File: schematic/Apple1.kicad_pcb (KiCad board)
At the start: 2 copper layers, 162.8 x 120.7 mm, 65 parts, among them J1 RCJ-041, J2 USB_A, J4 PWR, J5 ARM_JTAG_SWD, J6 SLOT, J7 EDGE, J8 12V, J9 -12V, SW1 RST, SW2 CLEAR, SW3 PWR, U1 WD65C02, U10 L7805, U2 6821 (W65C21N), U3 ATSAMD21E18A-A, U4 74LS138, U5 AT28C64B-15PU, U6 AS6C62256, U7 74HC00, U9 LD33CV

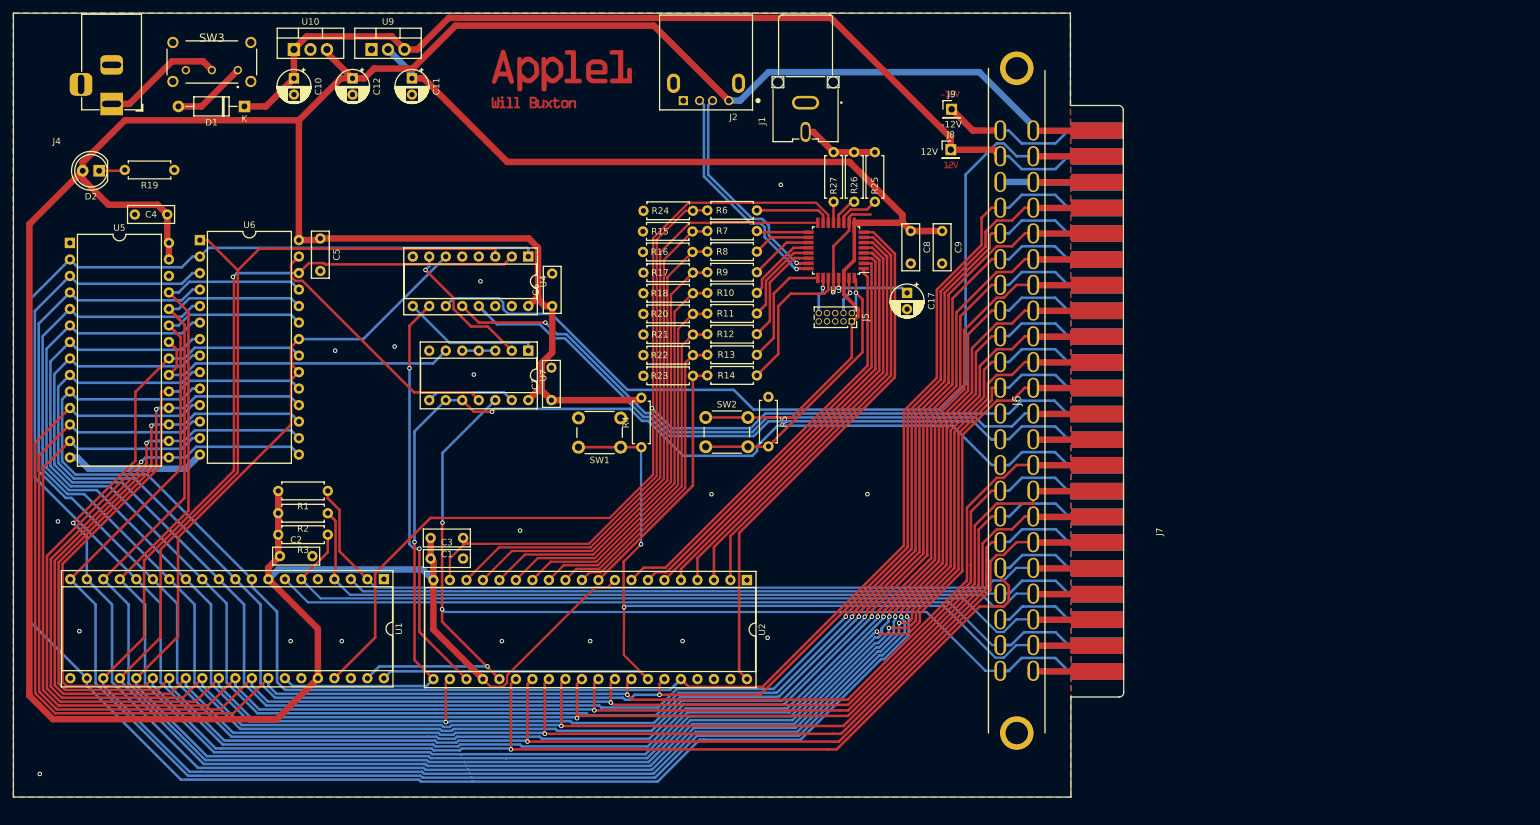
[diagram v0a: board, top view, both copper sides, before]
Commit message: rpi final
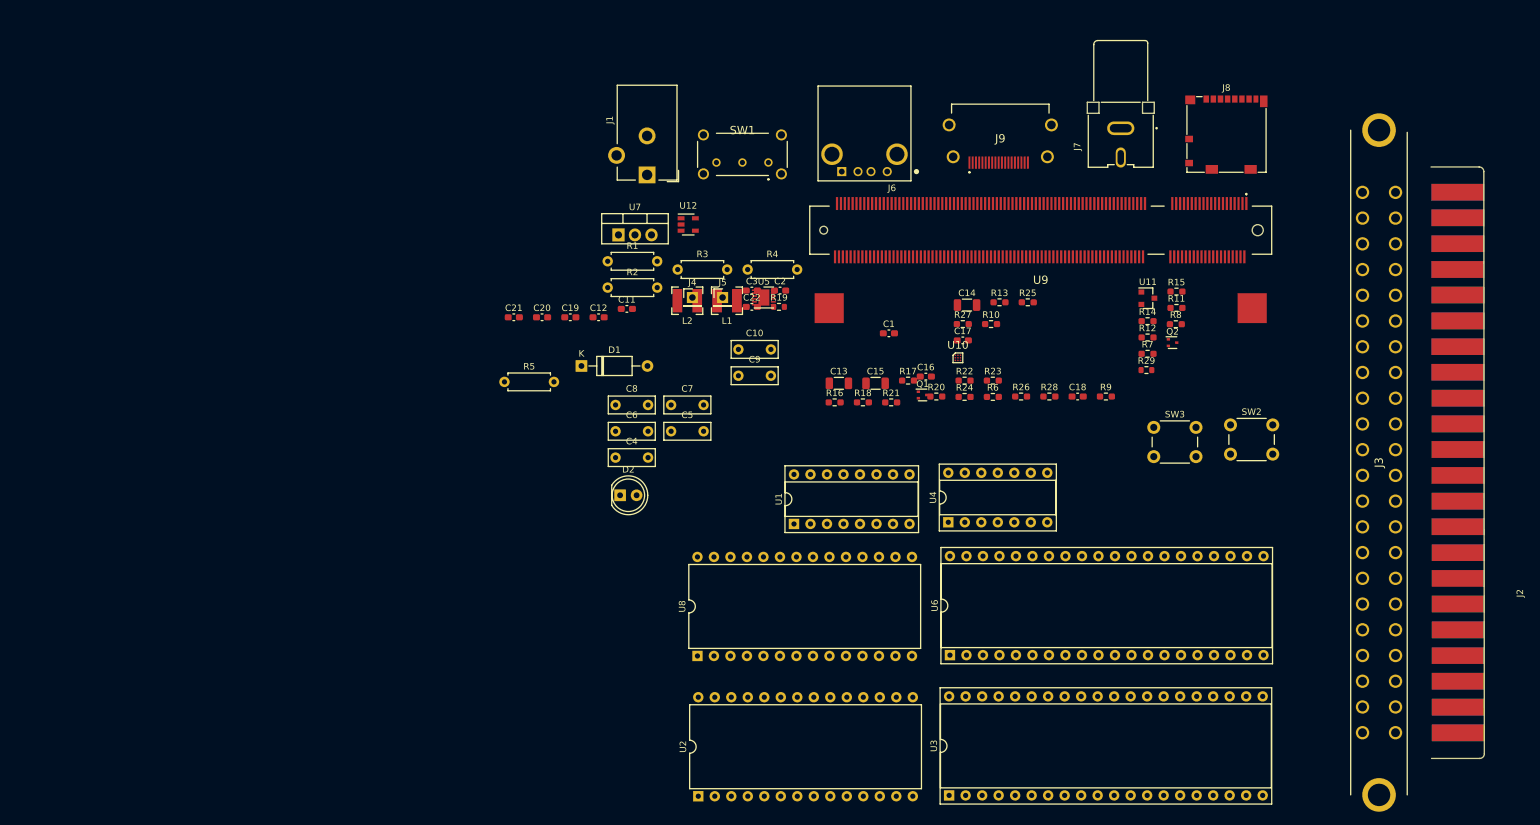
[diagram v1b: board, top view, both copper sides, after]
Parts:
- removed G***: LOGO, Apple1Title:n12v
- removed G***: LOGO, Apple1Title:12v
- removed G***: LOGO, Title:title
- added C13: 47uF, Capacitor_SMD:C_1206_3216Metric, F.Cu at (158.8, 74.6)
- added C14: 47uF, Capacitor_SMD:C_1206_3216Metric, F.Cu at (178.5, 62.6)
- added C15: 47uF, Capacitor_SMD:C_1206_3216Metric, F.Cu at (164.4, 74.6)
- added C16: 4.7uF, Capacitor_SMD:C_0603_1608Metric_Pad1.08x0.95mm_HandSolder, F.Cu at (172.2, 73.6)
- added C18: 0.1uF, Capacitor_SMD:C_0603_1608Metric_Pad1.08x0.95mm_HandSolder, F.Cu at (195.5, 76.7)
- added C19: 10uF, Capacitor_SMD:C_0603_1608Metric_Pad1.08x0.95mm_HandSolder, F.Cu at (117.5, 64.5)
- added C20: 10uF, Capacitor_SMD:C_0603_1608Metric_Pad1.08x0.95mm_HandSolder, F.Cu at (113.1, 64.5)
- added C21: 0.47uF, Capacitor_SMD:C_0603_1608Metric_Pad1.08x0.95mm_HandSolder, F.Cu at (108.8, 64.5)
- added C22: 0.47uF, Capacitor_SMD:C_0603_1608Metric_Pad1.08x0.95mm_HandSolder, F.Cu at (145.4, 62.9)
- added J3: SLOT, 307-044-520-202:307044520202, F.Cu at (244.5, 128.4)
- added L1: 4.7uH, Inductor_SMD:L_Bourns-SRN4018, F.Cu at (141.6, 61.9)
- added L2: 4.7uH, Inductor_SMD:L_Bourns-SRN4018, F.Cu at (135.5, 61.9)
- added Q1: DMG1012T, Package_TO_SOT_SMD:SOT-523, F.Cu at (171.7, 76.4)
- added Q2: DMG1012T, Package_TO_SOT_SMD:SOT-523, F.Cu at (210.2, 68.4)
- added R28: 2k, Resistor_SMD:R_0603_1608Metric_Pad0.98x0.95mm_HandSolder, F.Cu at (191.2, 76.7)
- added R29: 100k, Resistor_SMD:R_0603_1608Metric, F.Cu at (206.1, 72.6)
- added U11: AP2331W, Package_TO_SOT_SMD:SOT-23, F.Cu at (206.4, 61.5)
- added U12: AP7315DQ-2.5, Package_TO_SOT_SMD:SOT-23-5, F.Cu at (135.6, 50.2)
- added U8: AT28C64B-15PU, Package_DIP:DIP-28_W15.24mm, F.Cu at (137.0, 116.6)
- C1: value 0.01uF -> 0.33uF; footprint Capacitor_THT:C_Rect_L7.0mm_W2.5mm_P5.00mm -> Capacitor_SMD:C_0603_1608Metric_Pad1.08x0.95mm_HandSolder
- C10: value 10uF -> 0.1uF; footprint Capacitor_THT:CP_Radial_D5.0mm_P2.50mm -> Capacitor_THT:C_Rect_L7.0mm_W2.5mm_P5.00mm
- C11: footprint Capacitor_THT:CP_Radial_D5.0mm_P2.50mm -> Capacitor_SMD:C_0603_1608Metric_Pad1.08x0.95mm_HandSolder
- C12: value 1uF -> 10uF; footprint Capacitor_THT:CP_Radial_D5.0mm_P2.50mm -> Capacitor_SMD:C_0603_1608Metric_Pad1.08x0.95mm_HandSolder
- C17: value 1uF -> 0.1uF; footprint Capacitor_THT:CP_Radial_D5.0mm_P2.50mm -> Capacitor_SMD:C_0603_1608Metric_Pad1.08x0.95mm_HandSolder
- C2, C3: footprint Capacitor_THT:C_Rect_L7.0mm_W2.5mm_P5.00mm -> Capacitor_SMD:C_0603_1608Metric_Pad1.08x0.95mm_HandSolder
- C4: value 0.1uF -> 0.01uF
- J1: value RCJ-041 -> PWR; footprint CUI_RCJ-041 -> Connector_BarrelJack:BarrelJack_CUI_PJ-102AH_Horizontal
- J2: value USB_A -> EDGE; footprint UJ2-AH-4-TH:CUI_UJ2-AH-4-TH -> Connector_PCBEdge:EDAC_Edge_307-044-520-202
- J4: value PWR -> 12V; footprint Connector_BarrelJack:BarrelJack_Horizontal -> Connector_PinHeader_2.54mm:PinHeader_1x01_P2.54mm_Vertical
- J5: value ARM_JTAG_SWD -> -12V; footprint Connector_PinSocket_1.27mm:PinSocket_2x05_P1.27mm_Vertical -> Connector_PinHeader_2.54mm:PinHeader_1x01_P2.54mm_Vertical
- J6: value SLOT -> USB_A; footprint 307-044-520-202:307044520202 -> UJ2-AH-4-TH:CUI_UJ2-AH-4-TH
- J7: value EDGE -> RCJ-041; footprint Connector_PCBEdge:EDAC_Edge_307-044-520-202 -> CUI_RCJ-041
- J8: value 12V -> Micro_SD_Card_Det; footprint Connector_PinHeader_2.54mm:PinHeader_1x01_P2.54mm_Vertical -> Connector_Card:microSD_HC_Molex_104031-0811
- J9: value -12V -> HDMI_A; footprint Connector_PinHeader_2.54mm:PinHeader_1x01_P2.54mm_Vertical -> 10029449-111RLF:10029449111RLF
- R10, R11, R12, R13, R14, R6, R7, R8, R9: value 1K -> 2k; footprint Resistor_THT:R_Axial_DIN0207_L6.3mm_D2.5mm_P7.62mm_Horizontal -> Resistor_SMD:R_0603_1608Metric_Pad0.98x0.95mm_HandSolder
- R15, R16, R17, R18, R20, R21, R22, R23, R24: value 2k -> 1K; footprint Resistor_THT:R_Axial_DIN0207_L6.3mm_D2.5mm_P7.62mm_Horizontal -> Resistor_SMD:R_0603_1608Metric_Pad0.98x0.95mm_HandSolder
- R19: value 330 -> 100k; footprint Resistor_THT:R_Axial_DIN0207_L6.3mm_D2.5mm_P7.62mm_Horizontal -> Resistor_SMD:R_0603_1608Metric
- R25: footprint Resistor_THT:R_Axial_DIN0207_L6.3mm_D2.5mm_P7.62mm_Horizontal -> Resistor_SMD:R_0603_1608Metric_Pad0.98x0.95mm_HandSolder
- R26: value 560 -> 100k; footprint Resistor_THT:R_Axial_DIN0207_L6.3mm_D2.5mm_P7.62mm_Horizontal -> Resistor_SMD:R_0603_1608Metric_Pad0.98x0.95mm_HandSolder
- R27: value 220 -> 100k; footprint Resistor_THT:R_Axial_DIN0207_L6.3mm_D2.5mm_P7.62mm_Horizontal -> Resistor_SMD:R_0603_1608Metric_Pad0.98x0.95mm_HandSolder
- R5: value 3.3K -> 330
- SW1: value RST -> PWR; footprint Button_Switch_THT:SW_PUSH_6mm -> EG1224:EG1224
- SW2: value CLEAR -> RST
- SW3: value PWR -> CLEAR; footprint EG1224:EG1224 -> Button_Switch_THT:SW_PUSH_6mm
- U1: value WD65C02 -> 74LS138; footprint Package_DIP:DIP-40_W15.24mm_Socket -> Package_DIP:DIP-16_W7.62mm_Socket
- U10: value L7805 -> ESD5384; footprint Package_TO_SOT_THT:TO-220-3_Vertical -> SW-On-Semi:WLCSP9-1.14x1.14mm
- U2: value 6821 (W65C21N) -> AS6C62256; footprint Package_DIP:DIP-40_W15.24mm_Socket -> Package_DIP:DIP-28_W15.24mm
- U3: value ATSAMD21E18A-A -> WD65C02; footprint Package_QFP:TQFP-32_7x7mm_P0.8mm -> Package_DIP:DIP-40_W15.24mm_Socket
- U4: value 74LS138 -> 74HC00; footprint Package_DIP:DIP-16_W7.62mm_Socket -> Package_DIP:DIP-14_W7.62mm_Socket
- U5: value AT28C64B-15PU -> PAM2306AYPKE; footprint Package_DIP:DIP-28_W15.24mm -> Package_DFN_QFN:WDFN-12-1EP_3x3mm_P0.45mm_EP1.7x2.5mm
- U6: value AS6C62256 -> 6821 (W65C21N); footprint Package_DIP:DIP-28_W15.24mm -> Package_DIP:DIP-40_W15.24mm_Socket
- U7: value 74HC00 -> L7805; footprint Package_DIP:DIP-14_W7.62mm_Socket -> Package_TO_SOT_THT:TO-220-3_Vertical
- U9: value LD33CV -> RaspberryPi-CM3+L; footprint Package_TO_SOT_THT:TO-220-3_Vertical -> 1717254-4:17172544
- moved SW3 151.3 mm to (207.3, 81.4), turned to 0 degrees
- moved J2 143.0 mm to (263.1, 106.9), turned to 90 degrees
- moved U6 131.9 mm to (175.9, 116.5), turned to 90 degrees
- moved U10 112.7 mm to (177.1, 70.7)
- moved U5 107.1 mm to (147.3, 61.4)
- moved U9 106.7 mm to (189.9, 51.1)
- moved R19 95.4 mm to (149.6, 62.9), turned to 0 degrees
- moved D2 94.5 mm to (125.1, 91.9), turned to 0 degrees
- moved J4 94.2 mm to (136.3, 61.4), turned to 0 degrees
- moved C2 87.2 mm to (149.8, 60.3)
- moved U3 85.7 mm to (175.8, 138.0), turned to 90 degrees
- moved R15 82.6 mm to (210.8, 60.5)
- moved SW2 80.8 mm to (219.1, 81.0)
- moved C10 80.1 mm to (143.3, 69.4), turned to 0 degrees
- moved J6 80.1 mm to (166.2, 42.0), turned to 180 degrees
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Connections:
- C1 pad 1: /CB2 -> +12V
- C1 pad 2: VCC -> GND
- C10 pad 1: +12V -> +5V
- C11 pad 1: +3V3 -> +5V
- C12 pad 1: VCC -> +5V
- C17 pad 1: Net-(C17-Pad1) -> +5V
- C2 pad 1: VCC -> GND
- C2 pad 2: GND -> Net-(C2-Pad2)
- C3 pad 1: VCC -> +5V
- C4 pad 1: VCC -> /CB2
- C4 pad 2: GND -> +5V
- C5 pad 1: VCC -> +5V
- C6 pad 1: VCC -> +5V
- C7 pad 1: VCC -> +5V
- C8 pad 1: +3V3 -> +5V
- C9 pad 1: +3V3 -> +5V
- D2 pad 2: VCC -> +5V
- J1 pad 1: GND -> Net-(J1-Pad1)
- J1 pad 2: Net-(J1-Pad2) -> GND
- J2 pad 1: VCC -> /RF
- J2 pad 2: /KEYD- -> /PHI2O
- J2 pad 3: /KEYD+ -> /RESET
- J2 pad 4: GND -> /SYNC
- J2 pad 5: GND -> /NMI
- J4 pad 1: Net-(J4-Pad1) -> +12V
- J5 pad 1: +3V3 -> -12V
- J6 pad 1: /RF -> +5V
- J6 pad 2: /PHI2O -> /RaspberryPi/USB_D-
- J6 pad 3: /RESET -> /RaspberryPi/USB_D+
- J6 pad 4: /SYNC -> GND
- J6 pad 5: /NMI -> GND
- J7 pad 1: /RF -> GND
- J7 pad 2: /PHI2O -> /RaspberryPi/TVDAC
- J8 pad 1: +12V -> /RaspberryPi/SDX_D2
- J9 pad 1: -12V -> /RaspberryPi/HDMI_D2_P
- R1 pad 2: VCC -> +5V
- R10 pad 1: Net-(R10-Pad1) -> GND
- R11 pad 1: Net-(R11-Pad1) -> GND
- R11 pad 2: /PB3 -> /PB5
- R12 pad 1: Net-(R12-Pad1) -> GND
- R12 pad 2: /PB2 -> /PB6
- R13 pad 1: Net-(R13-Pad1) -> GND
- R13 pad 2: /PB1 -> /DA
- R14 pad 1: Net-(R14-Pad1) -> GND
- R14 pad 2: /PB0 -> /CB2
- R15 pad 1: GND -> Net-(R15-Pad1)
- R15 pad 2: /DA -> /RESET
- R16 pad 1: GND -> Net-(R16-Pad1)
- R16 pad 2: /PB6 -> /PB0
- R17 pad 1: GND -> Net-(R17-Pad1)
- R17 pad 2: /PB5 -> /PB1
- R18 pad 1: GND -> Net-(R18-Pad1)
- R18 pad 2: /PB4 -> /PB2
- R19 pad 1: GND -> +5V
- R19 pad 2: Net-(D2-Pad1) -> Net-(C2-Pad2)
- R2 pad 2: VCC -> +5V
- R20 pad 1: GND -> Net-(R20-Pad1)
- R21 pad 1: GND -> Net-(R21-Pad1)
- R21 pad 2: /PB2 -> /PB4
- R22 pad 1: GND -> Net-(R22-Pad1)
- R22 pad 2: /PB1 -> /PB5
- R23 pad 1: GND -> Net-(R23-Pad1)
- R23 pad 2: /PB0 -> /PB6
- R24 pad 1: GND -> Net-(R24-Pad1)
- R24 pad 2: /CB2 -> /DA
- R25 pad 2: Net-(J1-Pad2) -> /CB2
- R26 pad 1: Net-(R26-Pad1) -> /STROBE
- R26 pad 2: Net-(J1-Pad2) -> GND
- R27 pad 1: Net-(R27-Pad1) -> /PA0
- R27 pad 2: Net-(J1-Pad2) -> GND
- R3 pad 2: VCC -> +5V
- R4 pad 2: VCC -> +5V
- R5 pad 2: /SWDIO -> Net-(D2-Pad1)
- R6 pad 1: Net-(R6-Pad1) -> GND
- R6 pad 2: /CB2 -> /PB0
- R7 pad 1: Net-(R7-Pad1) -> GND
- R7 pad 2: /DA -> /PB1
- R8 pad 1: Net-(R8-Pad1) -> GND
- R8 pad 2: /PB6 -> /PB2
- R9 pad 1: Net-(R9-Pad1) -> GND
- R9 pad 2: /PB5 -> /PB3
- SW1 pad 1: /RESET -> Net-(D1-Pad2)
- SW1 pad 2: GND -> Net-(J1-Pad1)
- SW2 pad 1: +3V3 -> /RESET
- SW2 pad 2: /SWDIO -> GND
- SW3 pad 1: Net-(D1-Pad2) -> GND
- SW3 pad 2: Net-(J4-Pad1) -> /RaspberryPi/CLEAR
- U1 pad 1: (no net) -> /A12
- U1 pad 10: /A1 -> /$D000
- U1 pad 11: /A2 -> /$C000
- U1 pad 12: /A3 -> /$B000
- U1 pad 13: /A4 -> /$A000
- U1 pad 14: /A5 -> (no net)
- U1 pad 15: /A6 -> (no net)
- U1 pad 16: /A7 -> +5V
- U1 pad 2: /RDY -> /A13
- U1 pad 3: /PHI1O -> /A14
- U1 pad 4: /IQR -> GND
- U1 pad 5: (no net) -> GND
- U1 pad 6: /NMI -> /A15
- U1 pad 7: /SYNC -> /$F000
- U1 pad 8: VCC -> GND
- U1 pad 9: /A0 -> /$E000
- U2 pad 1: GND -> /A14
- U2 pad 10: /PB0 -> /A0
- U2 pad 11: /PB1 -> /D0
- U2 pad 12: /PB2 -> /D1
- U2 pad 13: /PB3 -> /D2
- U2 pad 14: /PB4 -> GND
- U2 pad 15: /PB5 -> /D3
- U2 pad 16: /PB6 -> /D4
- U2 pad 17: /DA -> /D5
- U2 pad 18: /RDA -> /D6
- U2 pad 19: /CB2 -> /D7
- U2 pad 2: /PA0 -> /A12
- U2 pad 20: VCC -> /A15
- U2 pad 21: /RW -> /A10
- U2 pad 22: /A4 -> /A15
- U2 pad 23: /$D000 -> /A11
- U2 pad 24: VCC -> /A9
- U2 pad 25: /PHI2O -> /A8
- U2 pad 26: /D7 -> /A13
- U2 pad 27: /D6 -> /WE
- U2 pad 28: /D5 -> +5V
- U2 pad 3: /PA1 -> /A7
- U2 pad 4: /PA2 -> /A6
- U2 pad 5: /PA3 -> /A5
- U2 pad 6: /PA4 -> /A4
- U2 pad 7: /PA5 -> /A3
- U2 pad 8: /PA6 -> /A2
- U2 pad 9: VCC -> /A1
- U3 pad 1: /PA6 -> (no net)
- U3 pad 10: GND -> /A1
- U3 pad 11: Net-(R25-Pad1) -> /A2
- U3 pad 12: Net-(R26-Pad1) -> /A3
- U3 pad 13: Net-(R27-Pad1) -> /A4
- U3 pad 14: /PHI2 -> /A5
- U3 pad 15: Net-(R6-Pad1) -> /A6
- U3 pad 16: /RDA -> /A7
- U3 pad 17: Net-(R7-Pad1) -> /A8
- U3 pad 18: Net-(R8-Pad1) -> /A9
- U3 pad 19: Net-(R9-Pad1) -> /A10
- U3 pad 2: /PA5 -> /RDY
- U3 pad 20: Net-(R10-Pad1) -> /A11
- U3 pad 21: Net-(R11-Pad1) -> GND
- U3 pad 22: Net-(R12-Pad1) -> /A12
- U3 pad 23: /KEYD- -> /A13
- U3 pad 24: /KEYD+ -> /A14
- U3 pad 25: Net-(R13-Pad1) -> /A15
- U3 pad 26: /RST -> /D7
- U3 pad 27: Net-(R14-Pad1) -> /D6
- U3 pad 28: GND -> /D5
- U3 pad 29: Net-(C17-Pad1) -> /D4
- U3 pad 3: /PA4 -> /PHI1O
- U3 pad 30: +3V3 -> /D3
- U3 pad 31: /SWCLK -> /D2
- U3 pad 32: /SWDIO -> /D1
- U3 pad 4: /PA3 -> /IQR
- U3 pad 5: /PA2 -> (no net)
- U3 pad 6: /PA1 -> /NMI
- U3 pad 7: /PA0 -> /SYNC
- U3 pad 8: /STROBE -> +5V
- U3 pad 9: +3V3 -> /A0
- U4 pad 1: /A12 -> /$E000
- U4 pad 10: /$D000 -> /RW
- U4 pad 11: /$C000 -> /WE
- U4 pad 12: /$B000 -> /PHI2O
- U4 pad 13: /$A000 -> Net-(U4-Pad13)
- U4 pad 14: (no net) -> +5V
- U4 pad 2: /A13 -> /$F000
- U4 pad 3: /A14 -> Net-(U4-Pad3)
- U4 pad 4: GND -> Net-(U4-Pad3)
- U4 pad 5: GND -> Net-(U4-Pad3)
- U4 pad 6: /A15 -> Net-(U4-Pad6)
- U4 pad 7: /$F000 -> GND
- U4 pad 8: GND -> Net-(U4-Pad13)
- U4 pad 9: /$E000 -> /RW
- U5 pad 1: (no net) -> +5V
- U5 pad 10: /A0 -> +1V8
- U5 pad 11: /D0 -> (no net)
- U5 pad 12: /D1 -> Net-(C2-Pad2)
- U5 pad 13: /D2 -> GND
- U5 pad 2: /A12 -> Net-(L2-Pad1)
- U5 pad 3: /A7 -> GND
- U5 pad 4: /A6 -> +3V3
- U5 pad 5: /A5 -> (no net)
- U5 pad 6: /A4 -> +5V
- U5 pad 7: /A3 -> +5V
- U5 pad 8: /A2 -> Net-(L1-Pad1)
- U5 pad 9: /A1 -> GND
- U6 pad 1: /A14 -> GND
- U6 pad 10: /A0 -> /PB0
- U6 pad 11: /D0 -> /PB1
- U6 pad 12: /D1 -> /PB2
- U6 pad 13: /D2 -> /PB3
- U6 pad 14: GND -> /PB4
- U6 pad 15: /D3 -> /PB5
- U6 pad 16: /D4 -> /PB6
- U6 pad 17: /D5 -> /DA
- U6 pad 18: /D6 -> /RDA
- U6 pad 19: /D7 -> /CB2
- U6 pad 2: /A12 -> /PA0
- U6 pad 20: /A15 -> +5V
- U6 pad 21: /A10 -> /RW
- U6 pad 22: /A15 -> /A4
- U6 pad 23: /A11 -> /$D000
- U6 pad 24: /A9 -> +5V
- U6 pad 25: /A8 -> /PHI2O
- U6 pad 26: /A13 -> /D7
- U6 pad 27: /WE -> /D6
- U6 pad 28: VCC -> /D5
- U6 pad 3: /A7 -> /PA1
- U6 pad 4: /A6 -> /PA2
- U6 pad 5: /A5 -> /PA3
- U6 pad 6: /A4 -> /PA4
- U6 pad 7: /A3 -> /PA5
- U6 pad 8: /A2 -> /PA6
- U6 pad 9: /A1 -> +5V
- U7 pad 1: /$E000 -> +12V
- U7 pad 2: /$F000 -> GND
- U7 pad 3: Net-(U7-Pad3) -> +5V
- U9 pad 2: +3V3 -> (no net)
- U9 pad 3: +12V -> Net-(R15-Pad1)
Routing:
- net VCC: track 553.1 -> 0.00 mm
- net /A12: track 352.5 -> 0.00 mm, vias 1 -> 0
- net /A14: track 316.7 -> 0.00 mm, vias 1 -> 0
- net /A13: track 315.8 -> 0.00 mm, vias 2 -> 0
- net /A11: track 292.3 -> 0.00 mm, vias 1 -> 0
- net /A7: track 290.1 -> 0.00 mm, vias 1 -> 0
- net /A9: track 289.3 -> 0.00 mm, vias 1 -> 0
- net /A4: track 288.2 -> 0.00 mm, vias 2 -> 0
- net /A8: track 287.7 -> 0.00 mm, vias 1 -> 0
- net /A6: track 287.7 -> 0.00 mm, vias 1 -> 0
- net /A15: track 287.2 -> 0.00 mm, vias 1 -> 0
- net /A10: track 284.0 -> 0.00 mm, vias 2 -> 0
- net /A5: track 283.3 -> 0.00 mm, vias 1 -> 0
- net /A3: track 276.8 -> 0.00 mm, vias 1 -> 0
- net /A2: track 274.9 -> 0.00 mm, vias 1 -> 0
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- removed copper zone on B.Cu, net GND
- removed copper zone on F.Cu, net GND
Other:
- board size 162.8 x 120.7 mm -> 8.2 x 91 mm
- copper layers 2 -> 4
- net class HDMI_dPair added: clearance 0.2, trace_width 0.2, via_dia 0.5, via_drill 0.2
- net class PWR added: clearance 0.2, trace_width 1, via_dia 1, via_drill 0.6
- net class Thic removed
- net class USB_dPair added: clearance 0.2, trace_width 0.2, via_dia 1, via_drill 0.6
- rule trace_min: 0.2 -> 0.1
- rule via_min_drill: 0.3 -> 0.127
- rule via_min_size: 0.4 -> 0.3
